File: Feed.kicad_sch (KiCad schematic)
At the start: 35 parts

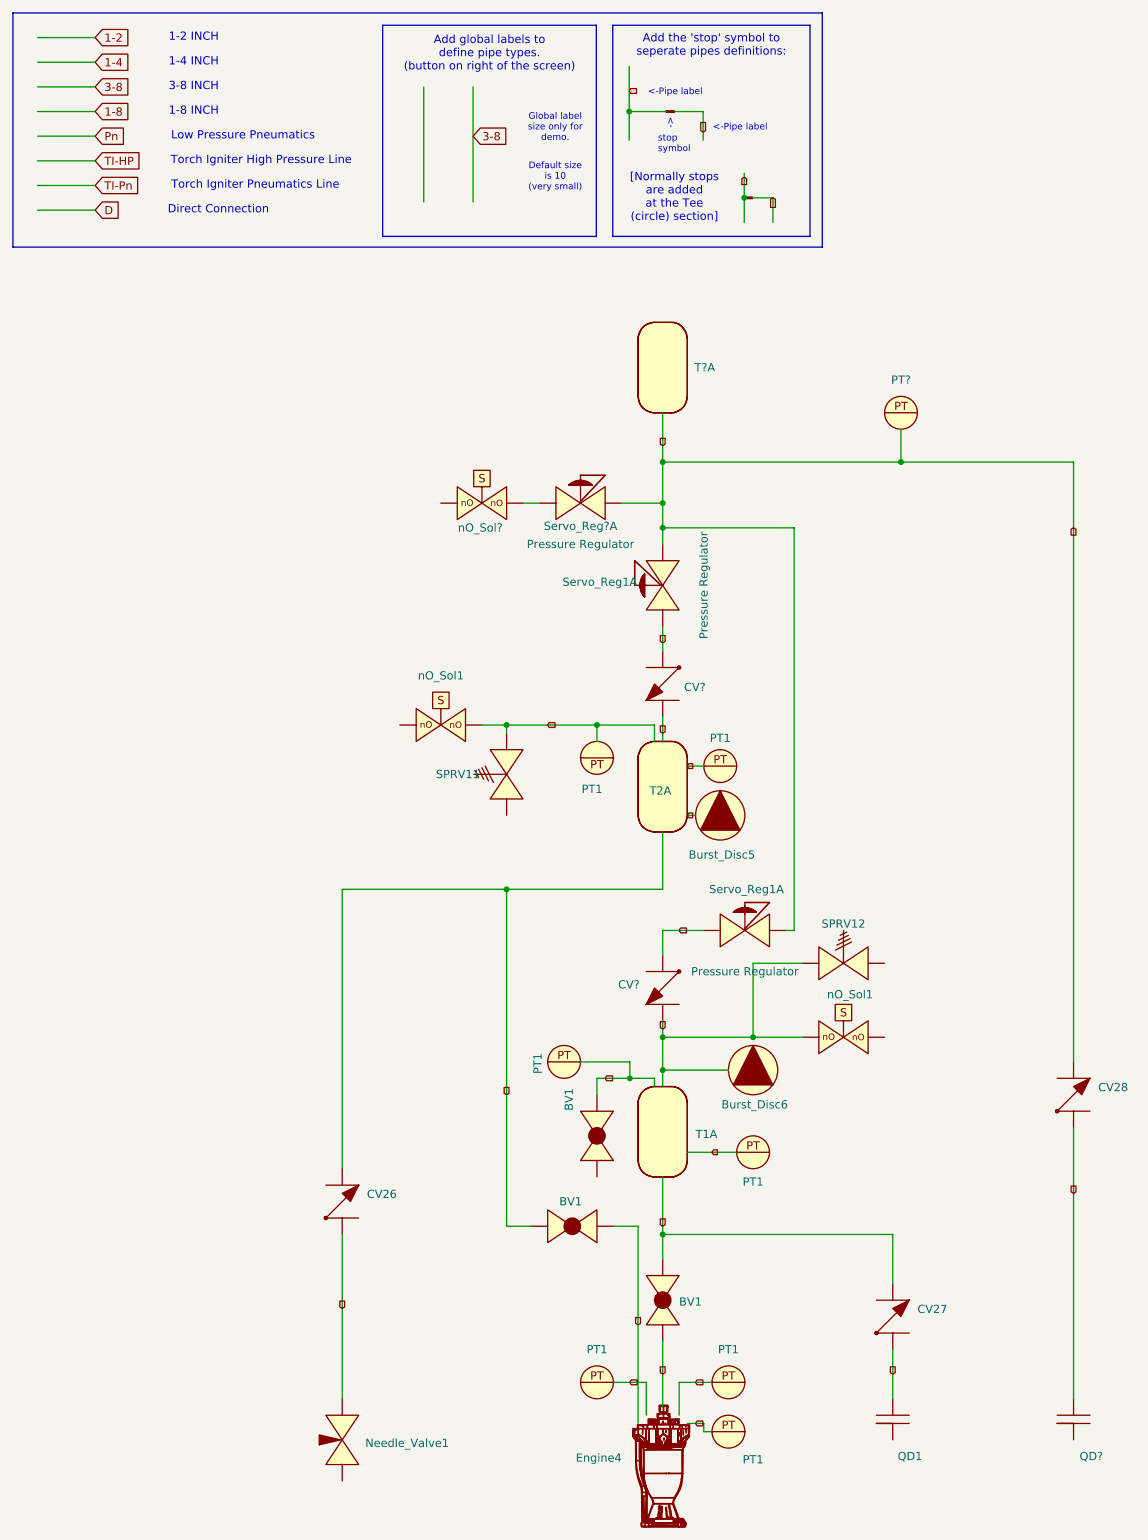
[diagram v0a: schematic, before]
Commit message: feed update
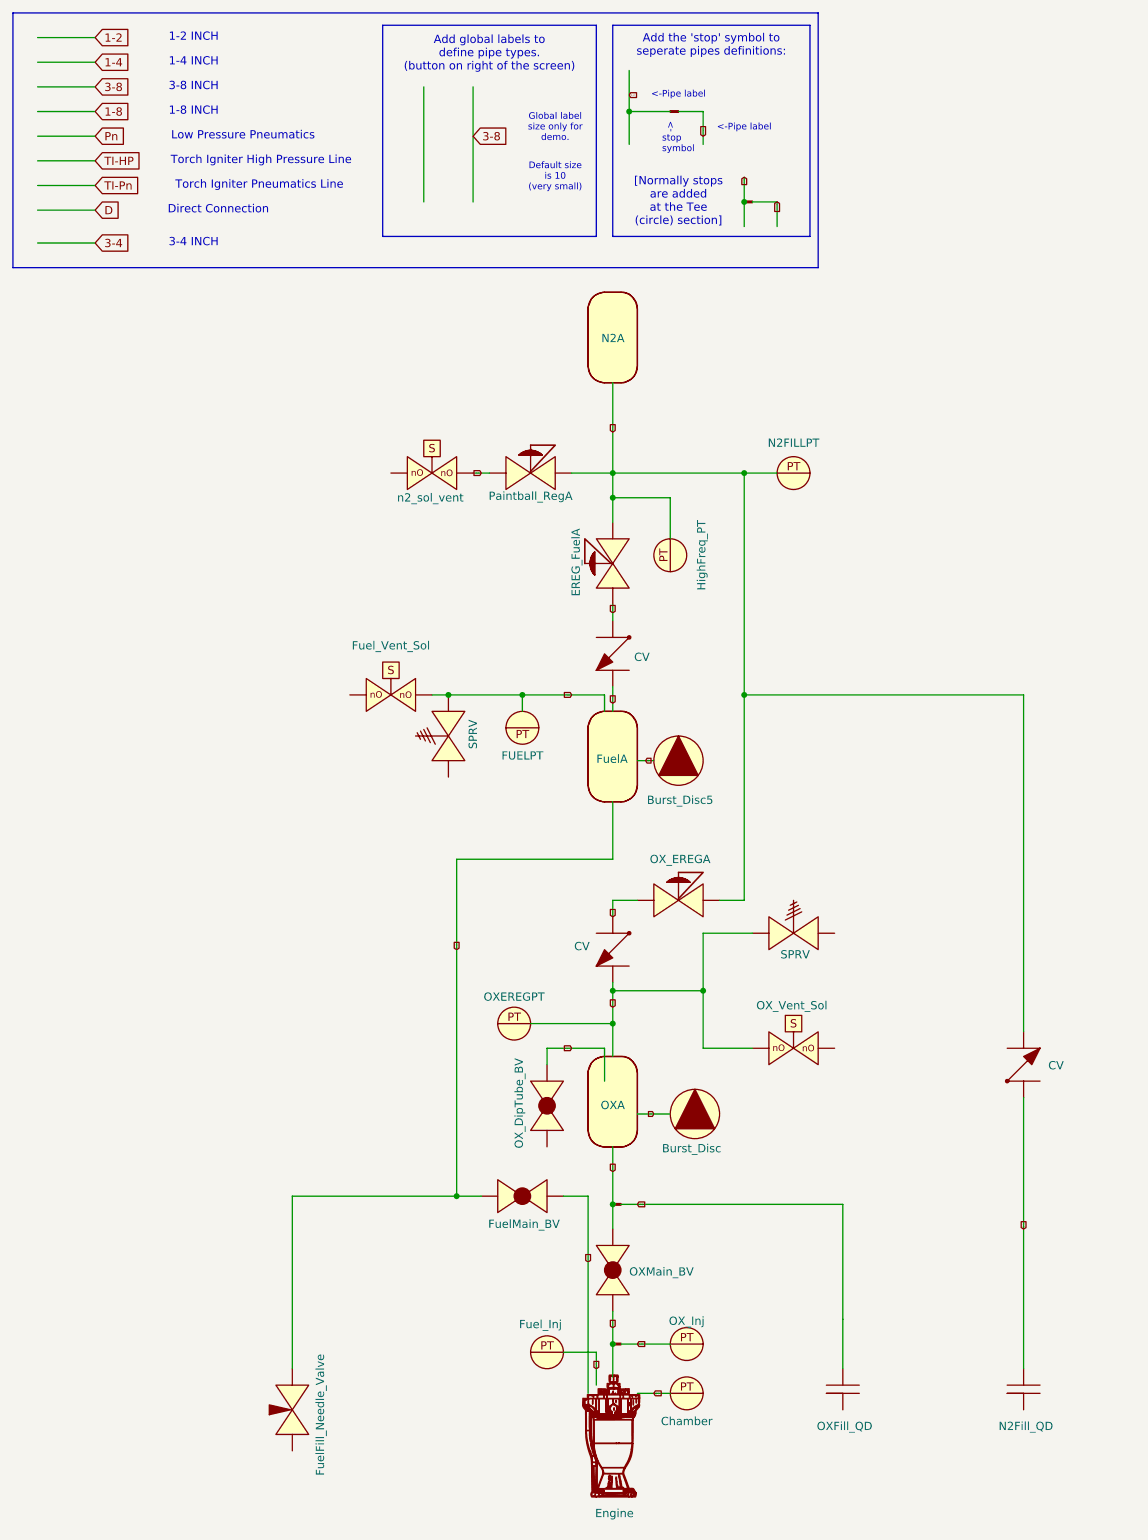
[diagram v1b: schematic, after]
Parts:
- removed CV26, CV27: ~, symbol PID_symbols:Check_Valve
- removed PT1 (x3): ~, symbol PID_symbols:Pressure_Transducer
- added HighFreq_PT, OX_Inj: ~, symbol PID_symbols:Pressure_Transducer
- added U72, U73: ~, symbol PID_symbols:stop
- gave numbers to parts that had none: 6
- renumbered Burst_Disc6 to Burst_Disc, CV28 to CV, PT1 to Chamber, Servo_Reg1 to EREG_Fuel, Engine4 to Engine, PT1 to FUELPT, T2 to Fuel, Needle_Valve1 to FuelFill_Needle_Valve, BV1 to FuelMain_BV, PT1 to Fuel_Inj, nO_Sol1 to Fuel_Vent_Sol, T1 to OX, PT1 to OXEREGPT, QD1 to OXFill_QD, BV1 to OXMain_BV, BV1 to OX_DipTube_BV, Servo_Reg1 to OX_EREG, nO_Sol1 to OX_Vent_Sol, SPRV12 to SPRV, SPRV11 to SPRV
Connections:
- net 1-2: now also FuelFill_Needle_Valve.
- net 1-4: now also n2_sol_vent., HighFreq_PT.; no longer Burst_Disc., CV., CV., Chamber., Engine., Fuel., FuelFill_Needle_Valve., Fuel_Inj., Fuel_Vent_Sol., OX., OXFill_QD., OX_Vent_Sol., SPRV., SPRV.
- net 3-4: now also U72., U73.
- net 3-8: now also CV., CV., EREG_Fuel., FUELPT., Fuel., Fuel_Vent_Sol., OX., OXEREGPT., OXFill_QD., OX_EREG., OX_Vent_Sol., SPRV., SPRV., U72.
- net D: now also Burst_Disc.; no longer FUELPT., OXEREGPT.
- net 1-8: now reaches Fuel_Inj.
- net 1-8: now also Chamber., Engine., OX_Inj., U73.
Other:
- note added: "3-4 INCH"
- moved on the sheet: Burst_Disc, Burst_Disc5, CV, Chamber, EREG_FuelA, Engine, FUELPT, FuelA, FuelFill_Needle_Valve, FuelMain_BV, Fuel_Inj, Fuel_Vent_Sol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
